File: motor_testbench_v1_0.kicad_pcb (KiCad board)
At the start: 4 copper layers, 99.5 x 74.5 mm, 252 parts, among them IC1 PJA3402_R1_00001, IC2 VIA2000SD, IC3 MIE1W0505BGLVH-3R-P, IC4 MCP3564RT-E_ST, J1 Conn_01x05_Pin, J10 Conn_01x02_Pin, J11 Conn_01x02_Pin, J12 Conn_01x02_Pin, J13 Conn_01x04_Pin, J2 Conn_01x01_Pin, J3 Conn_01x01_Pin, J4 Conn_01x22_Pin, J7 V_bat_in, J8 V_bat_out, J9 V_bat_secondary, U10 NCV8114BSN330T1G, U11 TPS7A2055PDBVR, U12 TLV75733PDYDR, U13 TPS7A2050PDBVR, U14 TPS7A2033PDBVR, U15 TPS7A2018PDBVRG4, U16 TPS7A2050PDBVR, U18 TPS7A2033PDBVR, U19 TPS7A2045PDBVR, U3 CZ3A05, U4 OPA2328DR, U5 OPA2328DR, U6 MCP1502T-50E/CHY, U7 TPS62933, U8 TPS62933, U9 OPA2387DR

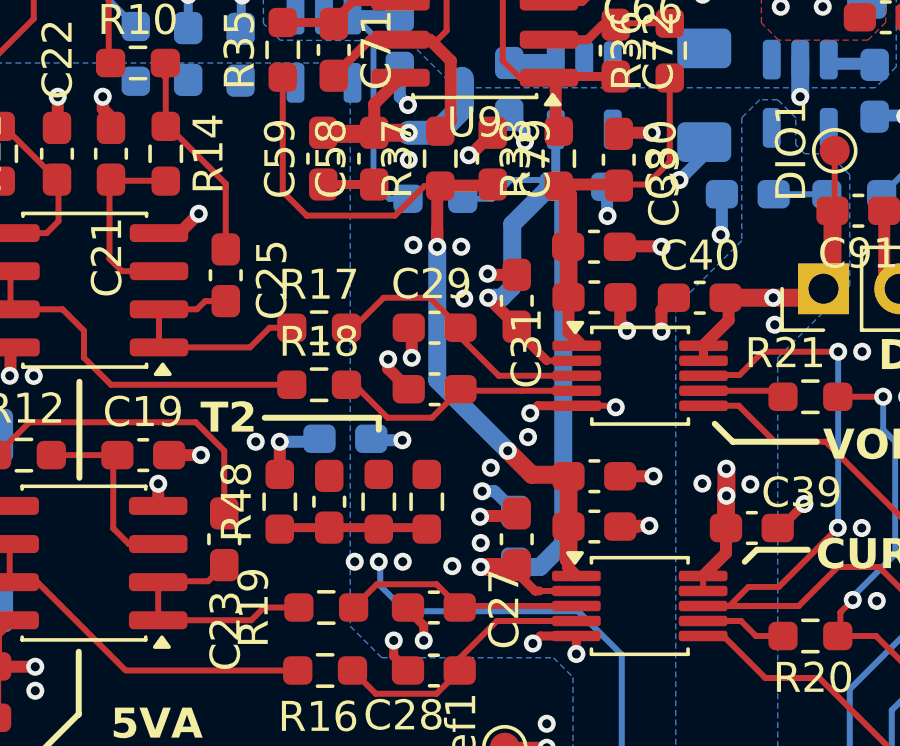
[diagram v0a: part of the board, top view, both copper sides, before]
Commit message: Minor fixes.
[KiCad Version: 10.0.4]
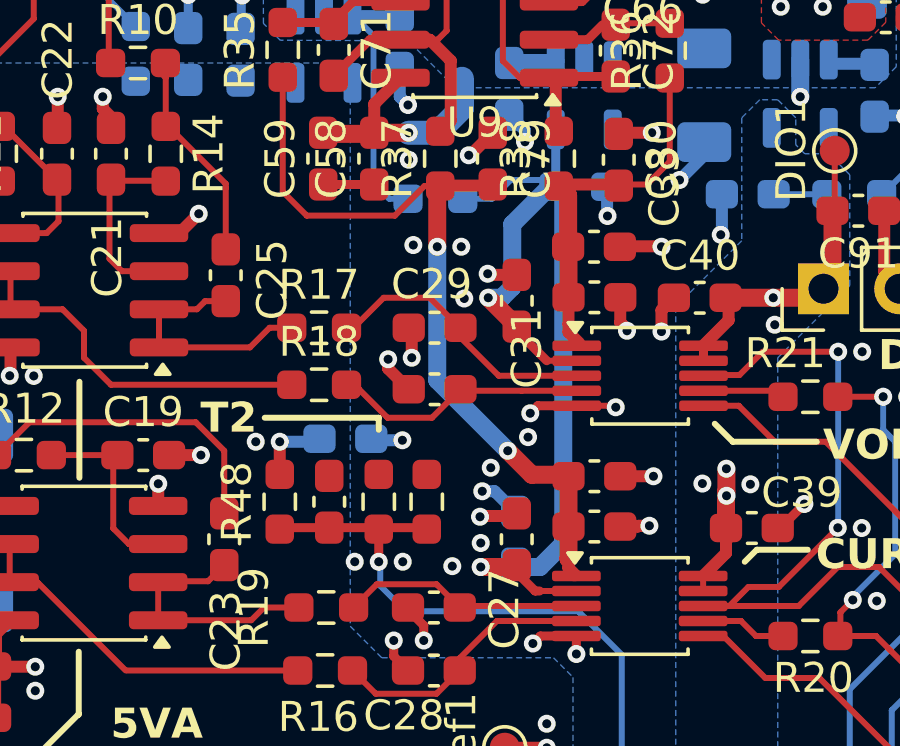
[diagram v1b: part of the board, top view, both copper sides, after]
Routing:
- net /Load Cell and Temperature Measurements/NTC_2: track 35.3 -> 36.4 mm
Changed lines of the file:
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@@
 		(start 136.4 76.15)
 		(end 135.45 75.2)
-		(width 0.4)
+		(width 0.6)
 		(layer "F.Cu")
 		(net "+1V8_MCP_AVIN")
@@
 		(start 133.749997 73.5)
 		(end 133.749997 71.575003)
-		(width 0.4)
+		(width 0.6)
 		(layer "F.Cu")
 		(net "+SAR_1_5V_Ref")
@@
 		(width 0.3)
 		(layer "F.Cu")
+		(net "/Load Cell and Temperature Measurements/NTC_2")
+	)
+	(segment
+		(start 131.8 84)
+		(end 131.8 82.9125)
+		(width 0.3)
+		(layer "F.Cu")
